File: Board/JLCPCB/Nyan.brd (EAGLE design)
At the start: 86 x 26 mm, 64 parts, among them IC1 74HCT541PW, IC2 STM32F10XCXT6, IC3 74HCT541PW, IC4 ST3485, U2 A4988_STEP, U3 MAX6966, X1 WR-WTB2.0-2_THT-VER, X10 32768, X2 WR-WTB2.0-4_THT_VER, X3 WR-WTB2.0-5_THT-VER, X4 WR-WTB2.0-5_THT-VER, X6 68610614122, X7 68612414422, X8 68610414122, X9 8M

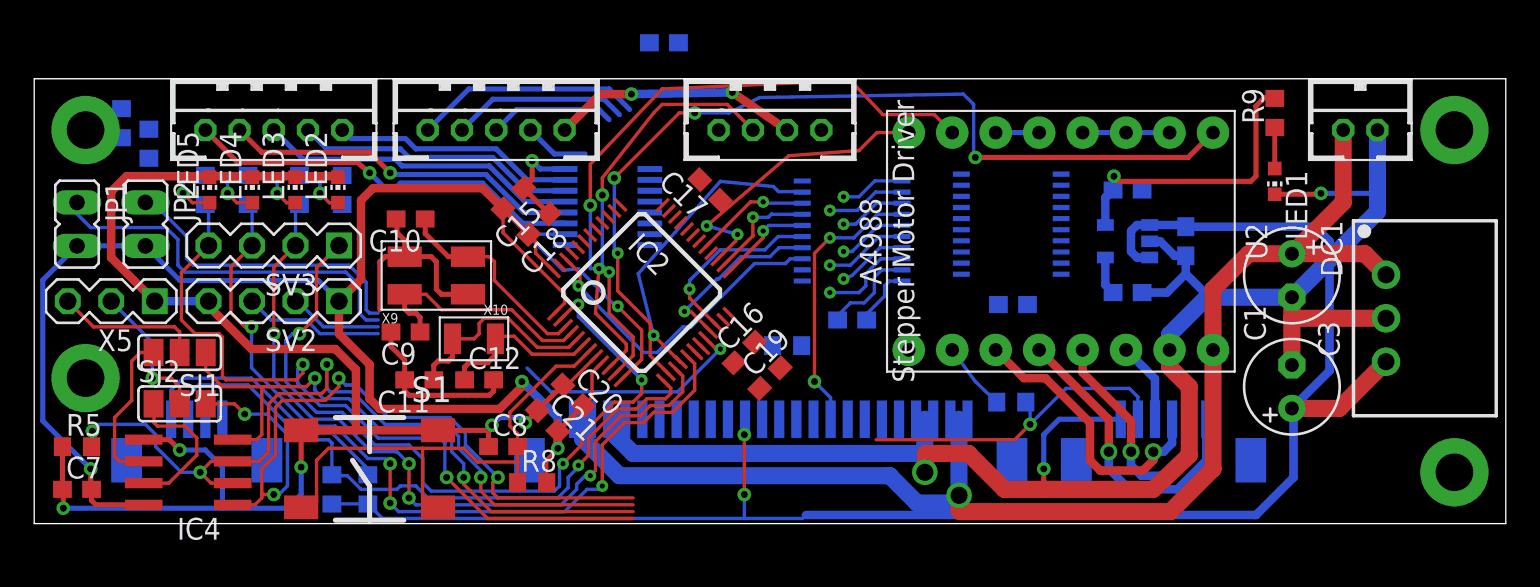
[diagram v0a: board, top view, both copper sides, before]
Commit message: [Board] More layouting done
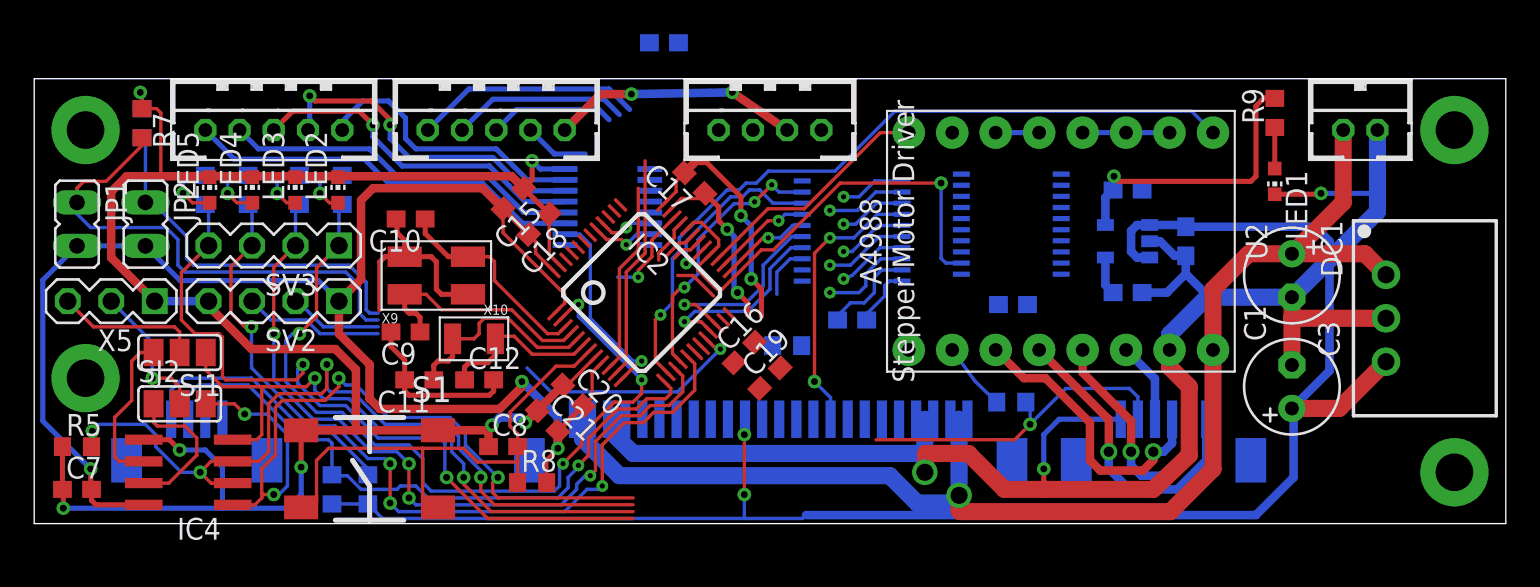
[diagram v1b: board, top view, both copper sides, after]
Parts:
- moved R6 1.26 mm to (6.30, 23.4), turned to 270 degrees
- moved R7 1.20 mm to (6.30, 23.4), flipped to the top, turned to 270 degrees
- moved C17 0.98 mm to (38.6, 19.9)
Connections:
- net N$7 renamed BOOT0
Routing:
- net GND: track 229.4 -> 261.5 mm, vias 9 -> 12
- net LATCH: track 0.00 -> 27.6 mm, vias 0 -> 1
- net MOT_STP: track 37.9 -> 11.2 mm, vias 2 -> 0
- net +3V3: track 115.6 -> 129.9 mm, vias 4 -> 6
- net D2: track 18.9 -> 5.70 mm, vias 1 -> 0
- net BUT_SIG: track 24.1 -> 13.2 mm, vias 2 -> 0
- net MOT_EN: track 53.5 -> 43.7 mm, vias 4 -> 1
- net BOOT0: track 22.7 -> 28.8 mm
- net SWDIO: track 5.45 -> 11.1 mm, vias 0 -> 1
- net DCLK: track 6.80 -> 11.2 mm
- net BOOT1: track 32.1 -> 35.9 mm
- net LED_MOSI: track 0.00 -> 3.76 mm, vias 0 -> 1
- net LED4: track 16.5 -> 19.9 mm, vias 0 -> 2
- net MOT_DIR: track 17.6 -> 14.3 mm, vias 2 -> 0
- net LED_MISO: track 0.00 -> 3.23 mm, vias 0 -> 1
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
